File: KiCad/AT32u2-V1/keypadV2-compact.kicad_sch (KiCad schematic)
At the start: 70 parts, among them J1 USB4085-GF-A_REVB, J2 AVR-ISP-6, SW2 RotaryEncoder_Switch, U1 ATmega32U2-A, U2 USBLC6-2SC6, Y1 16MHz

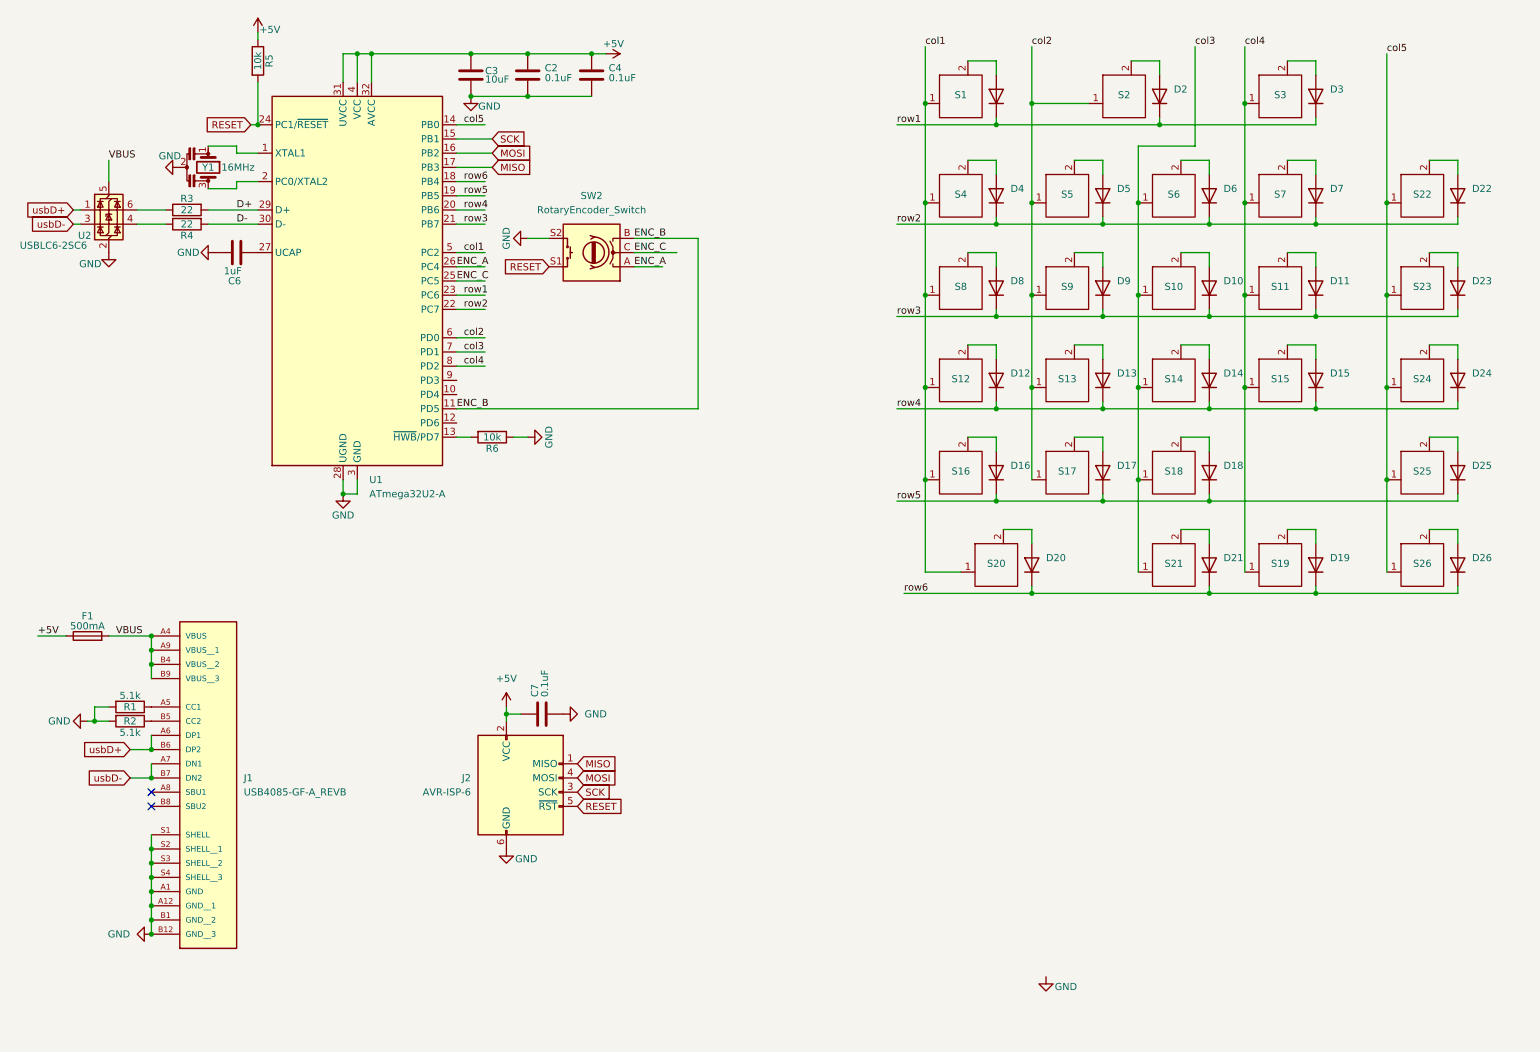
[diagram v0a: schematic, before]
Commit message: Schematic adjustment
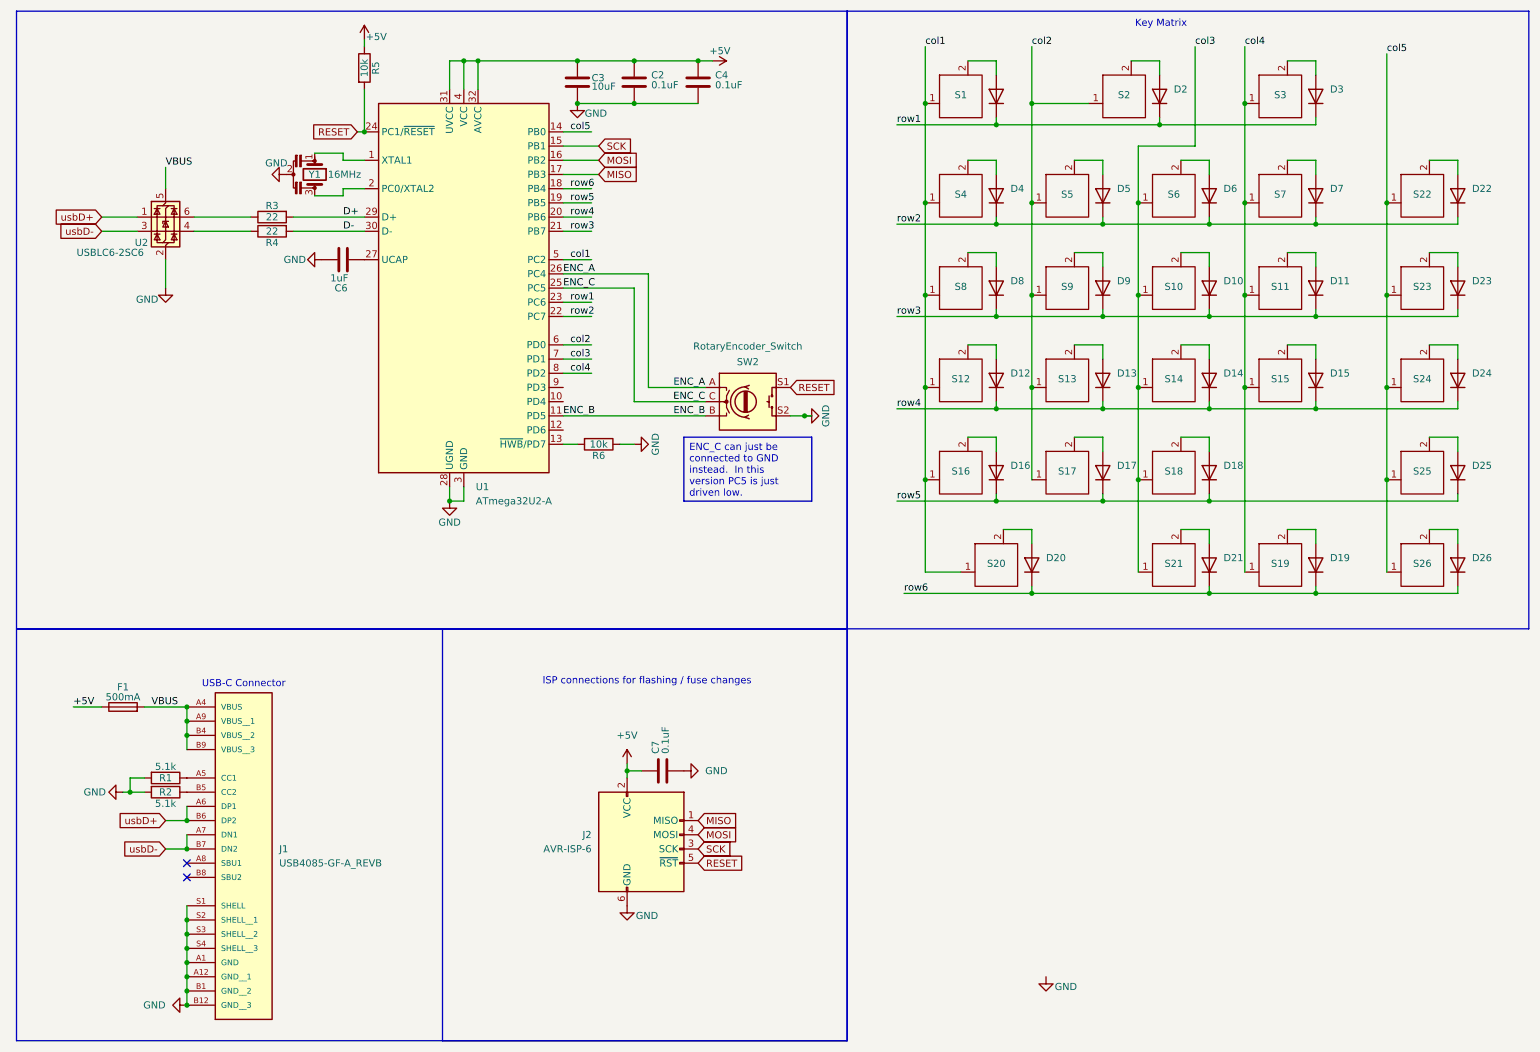
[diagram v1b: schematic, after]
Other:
- note added: "ISP connections for flashing / fuse changes"
- note added: "Key Matrix"
- note added: "USB-C Connector"
- moved on the sheet: C2, C3, C4, C6, C7, F1, J1, J2, R1, R2, R3, R4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
